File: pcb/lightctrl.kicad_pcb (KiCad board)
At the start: 2 copper layers, 76.8 x 36.8 mm, 30 parts, among them IC1 ESP-WROOM-02, P1 LED_CONN, P2 PROG, P3 IO, P4 BATT_SENSE, P5 5V, Q1 BSS138, Q2 IRF8788, SW1 SW_FLASH, SW2 SW_RST, U1 LM3940

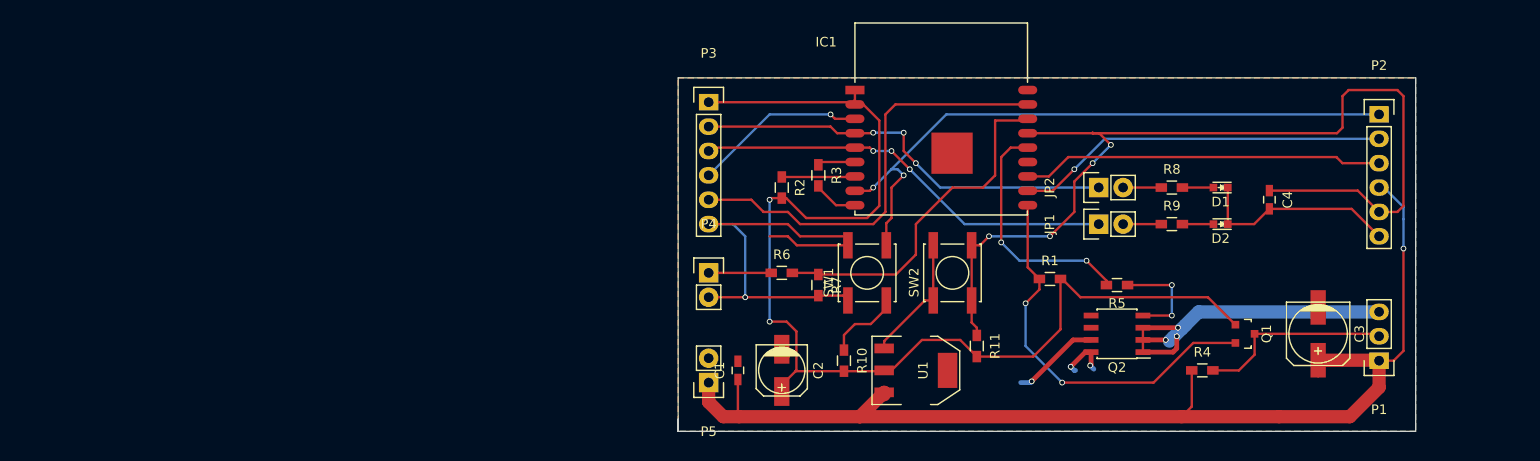
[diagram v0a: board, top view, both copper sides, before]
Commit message: New stick layout form
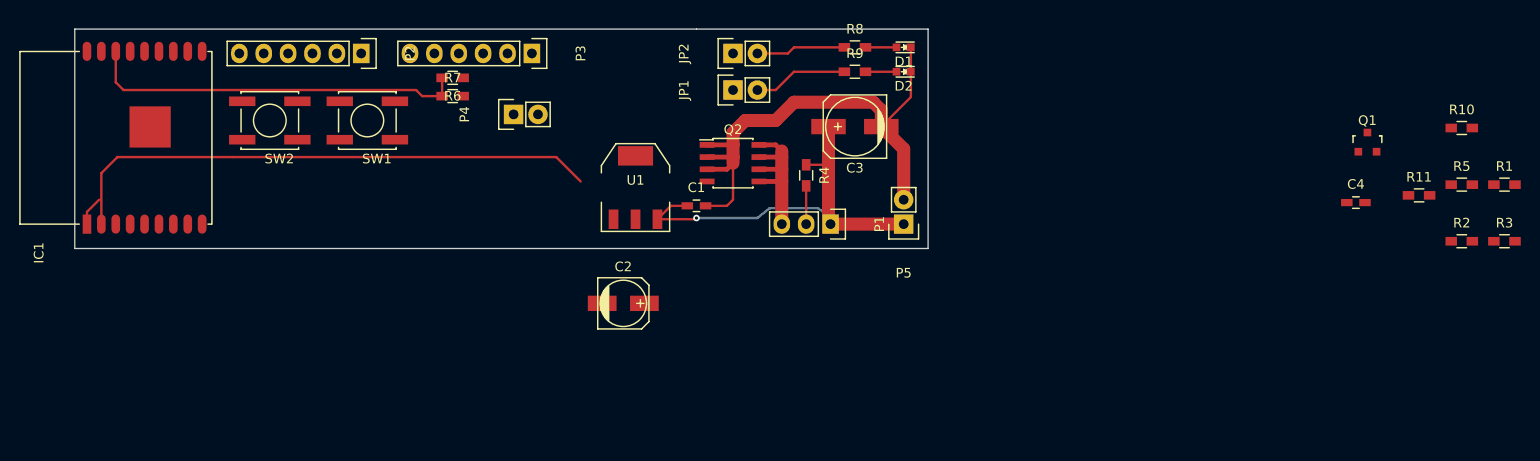
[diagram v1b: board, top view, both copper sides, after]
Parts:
- moved P2 106.2 mm to (107.3, 52.1), turned to 270 degrees
- moved IC1 81.2 mm to (78.7, 69.8), turned to 90 degrees
- moved SW2 72.9 mm to (97.8, 59.1), turned to 180 degrees
- moved R3 71.8 mm to (226.4, 71.6), turned to 0 degrees
- moved R2 71.1 mm to (222.0, 71.6), turned to 0 degrees
- moved R10 68.8 mm to (222.0, 59.8), turned to 0 degrees
- moved P1 58.9 mm to (156.2, 69.8), turned to 270 degrees
- moved SW1 54.4 mm to (108.0, 59.1), turned to 180 degrees
- moved C3 52.9 mm to (158.8, 59.7), turned to 180 degrees
- moved R11 48.7 mm to (217.5, 66.9), turned to 0 degrees
- moved R1 48.4 mm to (226.4, 65.7)
- moved R4 46.0 mm to (153.7, 64.8), turned to 270 degrees
- moved Q2 43.8 mm to (146.1, 63.5), turned to 0 degrees
- moved R7 42.9 mm to (116.8, 56.5), turned to 0 degrees
- moved JP1 40.6 mm to (146.1, 55.9)
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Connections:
- Q2 pad 1: Net-(P1-Pad3) -> GND
- Q2 pad 2: Net-(P1-Pad3) -> GND
- Q2 pad 3: Net-(P1-Pad3) -> GND
- Q2 pad 5: GND -> Net-(P1-Pad3)
- Q2 pad 6: GND -> Net-(P1-Pad3)
- Q2 pad 7: GND -> Net-(P1-Pad3)
- Q2 pad 8: GND -> Net-(P1-Pad3)
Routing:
- net /ESP8266/CTS: track 102.6 -> 0.00 mm, vias 4 -> 0
- net /ESP8266/BOOT_SEL: track 75.4 -> 0.00 mm, vias 2 -> 0
- net +5V: track 119.1 -> 44.2 mm
- net +3V3: track 120.5 -> 60.1 mm, vias 2 -> 0
- net GND: track 103.9 -> 55.4 mm, vias 4 -> 0
- net /ESP8266/IO16: track 45.4 -> 0.00 mm
- net /ESP8266/IO12: track 44.4 -> 0.00 mm, vias 3 -> 0
- net /ESP8266/IO13: track 44.1 -> 0.00 mm, vias 3 -> 0
- net /ESP8266/LED_DATA: track 40.9 -> 0.00 mm, vias 2 -> 0
- net /ESP8266/RXI: track 38.9 -> 0.00 mm, vias 1 -> 0
- net /ESP8266/TXO: track 37.7 -> 0.00 mm
- net /ESP8266/LED_PWR: track 25.1 -> 0.00 mm, vias 2 -> 0
- net Net-(P1-Pad3): track 39.4 -> 17.4 mm, vias 3 -> 0
- net /ESP8266/IO14: track 18.1 -> 0.00 mm, vias 1 -> 0
- net /ESP8266/WS2812_DATA: track 20.3 -> 3.98 mm
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- removed copper zone on B.Cu, net GND
- removed copper zone on F.Cu, net GND
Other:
- board size 76.8 x 36.8 mm -> 88.9 x 22.9 mm
- net class Default: clearance 0.2 -> 0.1524; trace_width 0.25 -> 0.1524; via_dia 0.6 -> 0.6858; via_drill 0.4 -> 0.3302
- rule trace_clearance: 0.2 -> 0.1524
- rule trace_min: 0.2 -> 0.1524
- rule via_min_drill: 0.3 -> 0.3302
- rule via_min_size: 0.4 -> 0.6858
